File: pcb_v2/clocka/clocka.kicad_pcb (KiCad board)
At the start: 2 copper layers, 114.3 x 125 mm, 63 parts, among them J2 control panel, J26 bus clock, J3 control panel, U1 74LS74, U10 74LS125, U11 NE555P, U12 NE555P, U2 74LS74, U3 74LS74, U4 74LS04, U5 74LS125, U6 74LS86, U7 74LS08, U8 NE555P, U9 NE555P, Y1 400KHz, Y2 1MHz

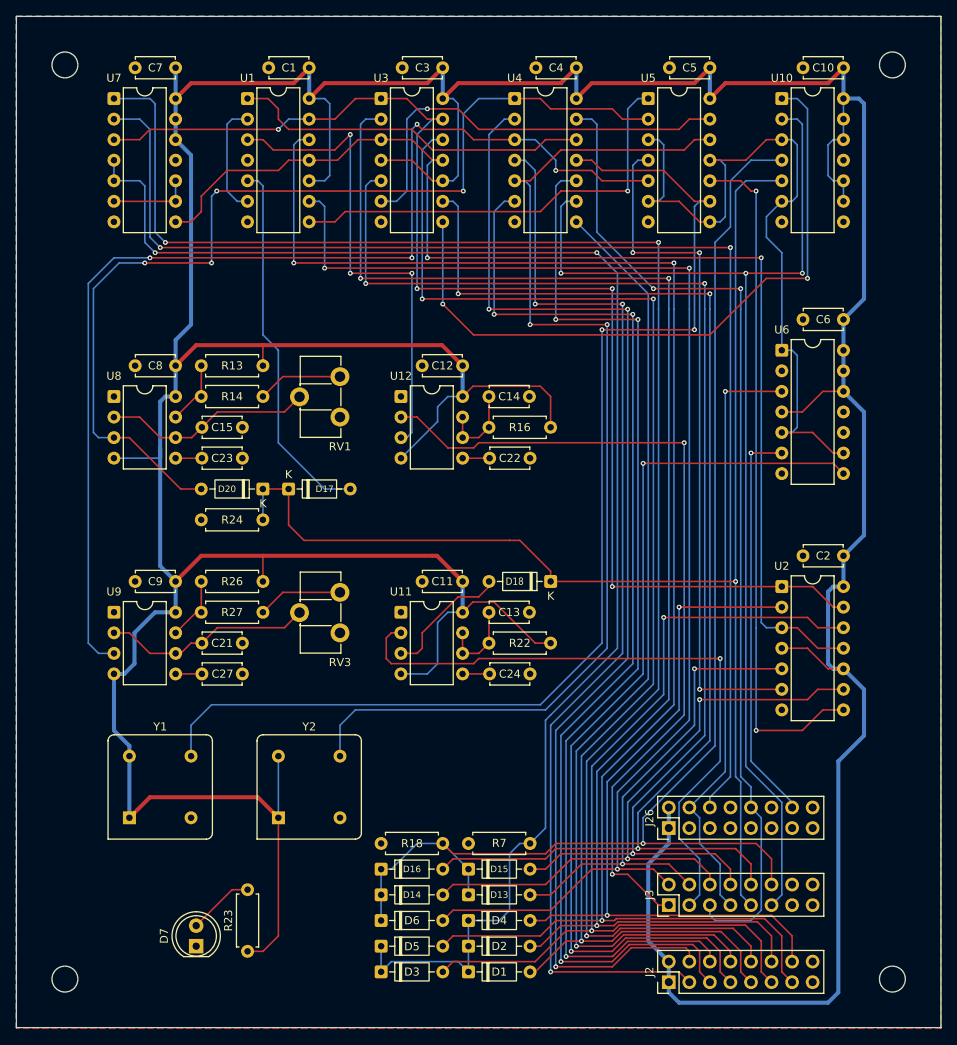
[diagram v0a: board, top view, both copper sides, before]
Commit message: novo layout do pcb
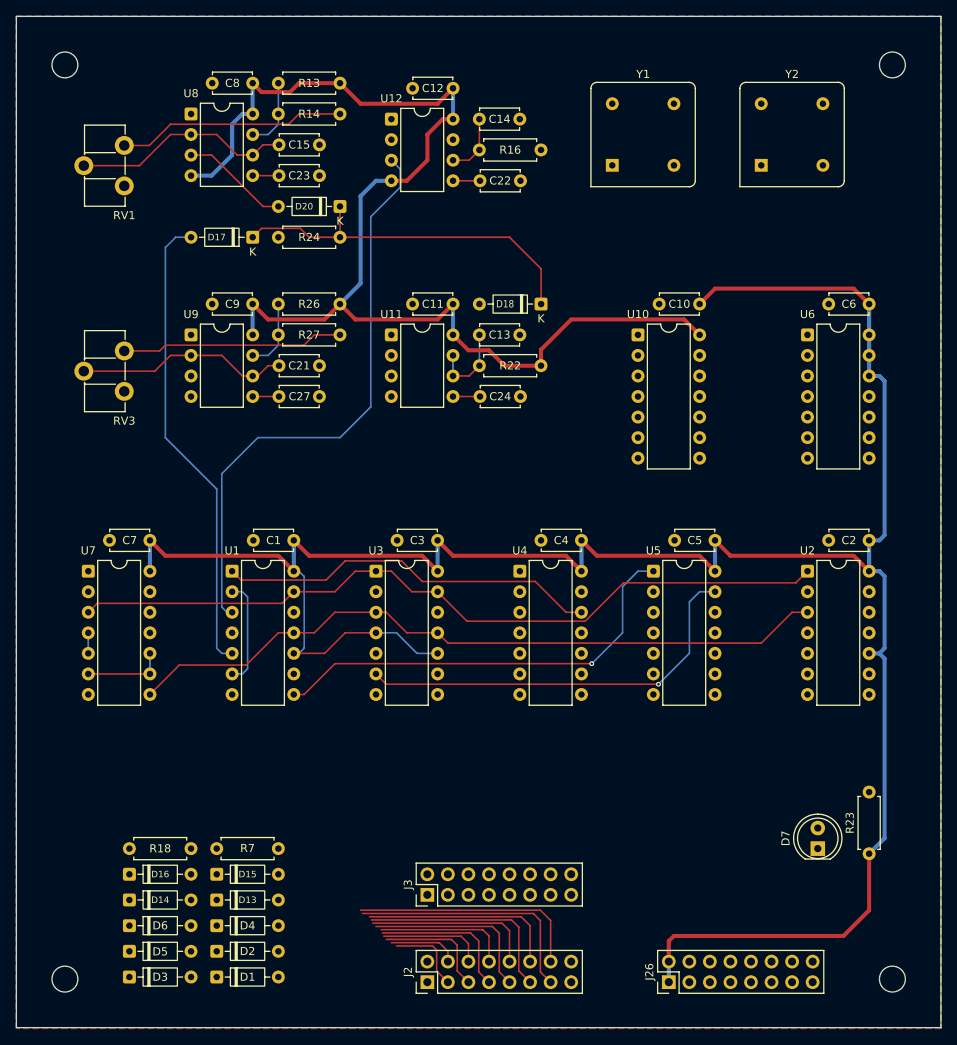
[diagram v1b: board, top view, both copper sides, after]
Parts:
- moved Y2 100.3 mm to (261.0, 47.0)
- moved Y1 100.3 mm to (242.6, 47.0)
- moved D7 77.8 mm to (268.0, 131.4)
- moved R23 77.8 mm to (274.3, 132.1)
- moved C7 58.5 mm to (180.4, 93.3)
- moved U7 58.5 mm to (177.8, 97.2)
- moved C1 58.5 mm to (198.2, 93.3)
- moved U1 58.5 mm to (195.6, 97.2)
- moved C4 58.4 mm to (233.8, 93.3)
- moved C5 58.4 mm to (250.3, 93.3)
- moved U4 58.4 mm to (231.1, 97.2)
- moved U5 58.4 mm to (247.7, 97.2)
- moved C3 58.4 mm to (216.0, 93.3)
- moved U3 58.4 mm to (213.4, 97.2)
- moved RV3 40.0 mm to (182.2, 74.9)
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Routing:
- net +5V: track 648.2 -> 435.5 mm
- net Net-(D1-K): track 185.6 -> 2.54 mm, vias 2 -> 0
- net ~{operator_break}: track 196.9 -> 21.1 mm, vias 3 -> 0
- net set_clock_1hz: track 199.2 -> 30.5 mm, vias 3 -> 0
- net clock_1hz: track 164.2 -> 0.00 mm, vias 3 -> 0
- net ~{clock_manual}: track 162.4 -> 0.00 mm, vias 1 -> 0
- net ~{control_break}: track 160.9 -> 0.00 mm, vias 2 -> 0
- net clock_ext: track 158.8 -> 0.00 mm, vias 3 -> 0
- net clock_xtal2: track 158.6 -> 0.00 mm, vias 3 -> 0
- net set_clock_xtal2: track 178.6 -> 24.8 mm, vias 3 -> 0
- net signal_xtal1: track 145.6 -> 0.00 mm, vias 2 -> 0
- net set_clock_ext: track 166.6 -> 22.2 mm, vias 3 -> 0
- net signal_ext: track 142.6 -> 0.00 mm, vias 3 -> 0
- net signal_1KHz: track 138.5 -> 0.00 mm, vias 4 -> 0
- net Net-(J2-Pin_4): track 146.6 -> 8.70 mm, vias 3 -> 0
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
